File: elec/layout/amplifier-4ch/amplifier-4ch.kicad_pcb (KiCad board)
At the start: 2 copper layers, 9 parts, among them U1 240kΩ ±1% 62.5mW, U2 33kΩ ±1% 62.5mW, U3 240kΩ ±1% 62.5mW, U4 33kΩ ±1% 62.5mW, U5 240kΩ ±1% 62.5mW, U6 33kΩ ±1% 62.5mW, U7 240kΩ ±1% 62.5mW, U8 33kΩ ±1% 62.5mW

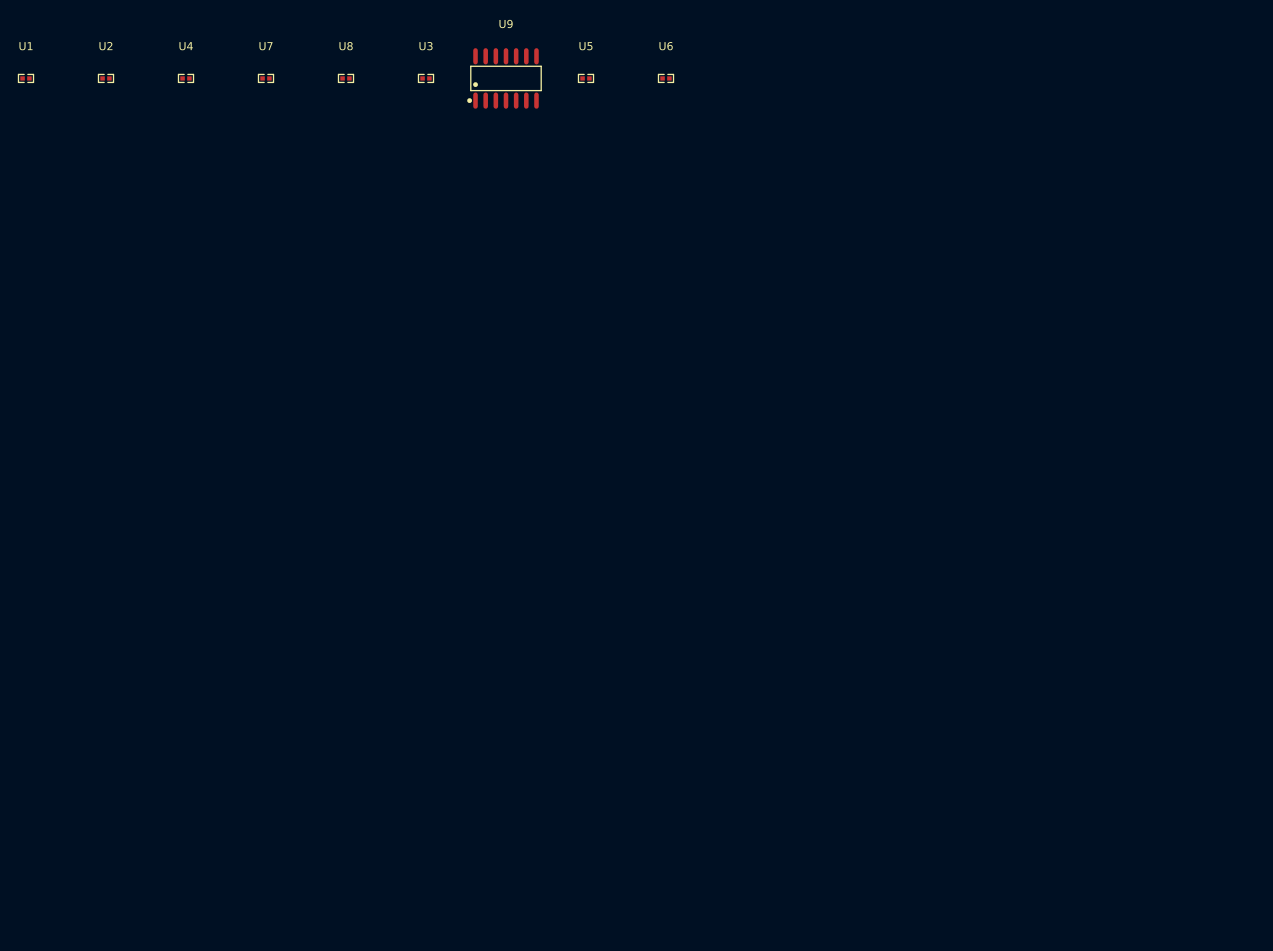
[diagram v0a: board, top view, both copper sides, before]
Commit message: Layout of amplifier-4ch
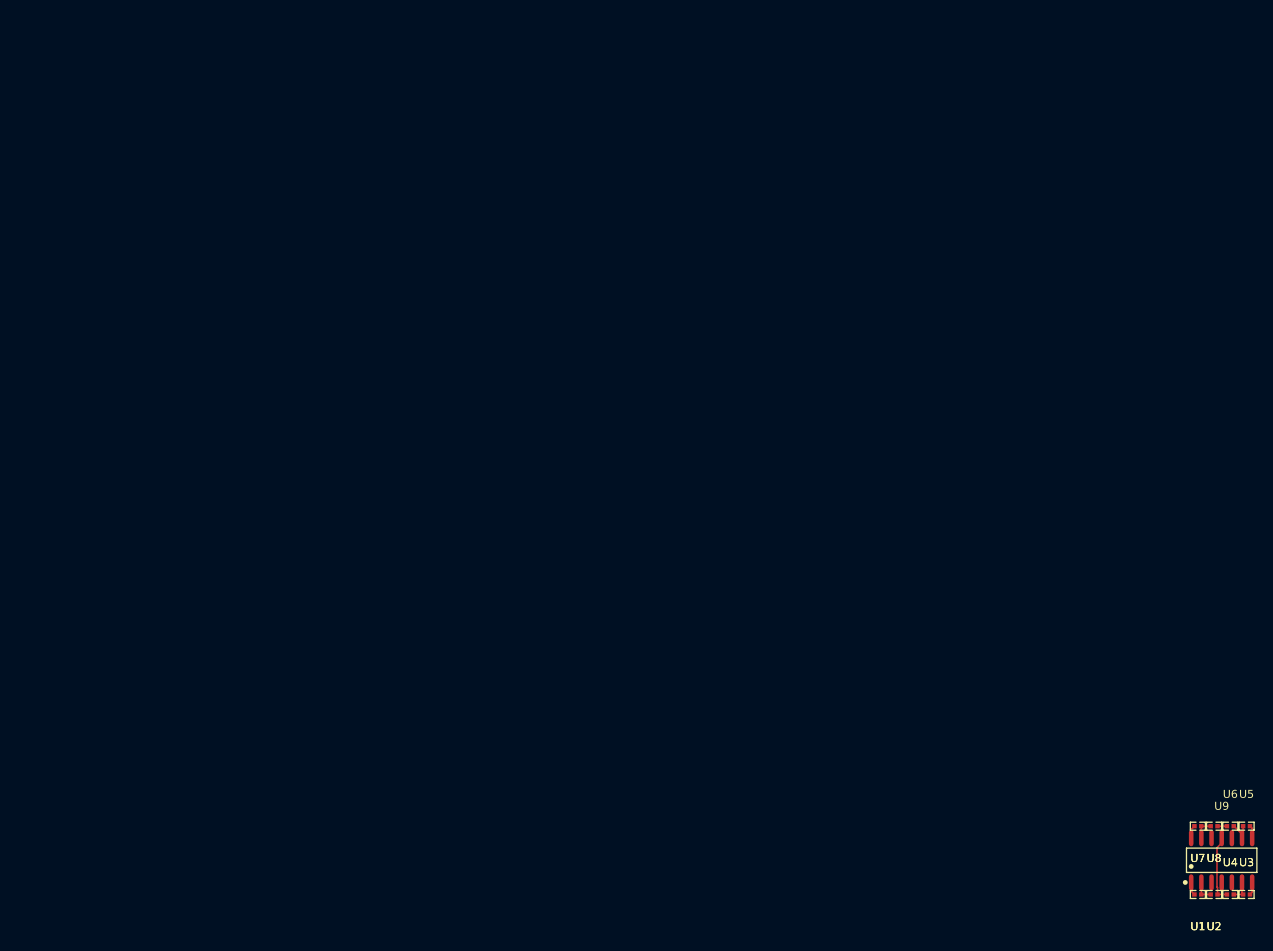
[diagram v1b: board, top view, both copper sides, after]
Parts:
- moved U1 178.5 mm to (156.5, 97.0), turned to 180 degrees
- moved U2 172.0 mm to (158.5, 97.0), turned to 180 degrees
- moved U4 165.7 mm to (160.5, 97.0)
- moved U7 149.3 mm to (156.5, 88.5), turned to 180 degrees
- moved U3 144.7 mm to (162.6, 97.0)
- moved U8 143.2 mm to (158.5, 88.5), turned to 180 degrees
- moved U9 132.5 mm to (159.5, 92.7)
- moved U5 124.7 mm to (162.6, 88.5)
- moved U6 117.1 mm to (160.5, 88.5)
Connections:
- net IN1_ renamed negative_terminal_1
- net IN1plus renamed input_1
- net IN2_ renamed negative_terminal_2
- net IN2plus renamed input_2
- net IN3_ renamed negative_terminal_3
- net IN4_ renamed negative_terminal_4
- net IN4plus renamed input_4
- net line renamed output_terminal_1
- net line-1 renamed output_terminal_2
- net line-2 renamed input_3
- net line-3 renamed output_terminal_4
- net line-4 renamed output_terminal_3
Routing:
- net gnd: track 0.00 -> 12.1 mm
- net negative_terminal_3: track 0.00 -> 3.49 mm
- net negative_terminal_2: track 0.00 -> 3.40 mm
- net negative_terminal_1: track 0.00 -> 3.18 mm
- net negative_terminal_4: track 0.00 -> 2.66 mm
- net output_terminal_4: track 0.00 -> 2.18 mm
- net output_terminal_1: track 0.00 -> 2.17 mm
- net output_terminal_2: track 0.00 -> 2.11 mm
- net output_terminal_3: track 0.00 -> 1.60 mm

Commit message: update syntax, delete vendored packages
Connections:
- net input_1 renamed IN1plus
- net input_2 renamed IN2plus
- net input_3 renamed IN3plus
- net input_4 renamed IN4plus
- net negative_terminal_1 renamed IN1_
- net negative_terminal_2 renamed IN2_
- net negative_terminal_3 renamed IN3_
- net negative_terminal_4 renamed IN4_
- net output_terminal_1 renamed line-2
- net output_terminal_2 renamed line-1
- net output_terminal_3 renamed line
- net output_terminal_4 renamed line-3

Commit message: build and re-link layouts
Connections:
- U3 pad 2: line-1 -> line
- U5 pad 2: line -> line-1
- U9 pad 7: line-1 -> line
- U9 pad 8: line -> line-1
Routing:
- net line-1: track 2.11 -> 1.60 mm
- net line: track 1.60 -> 2.11 mm
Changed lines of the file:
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@@
     (net 3 "IN2plus")
     (net 4 "IN1plus")
-    (net 5 "line")
+    (net 5 "line-1")
     (net 6 "hv")
     (net 7 "IN4plus")
@@
     (net 11 "line-2")
     (net 12 "IN4_")
-    (net 13 "line-1")
+    (net 13 "line")
     (net 14 "IN1_")
     (footprint "atopile:R0402-56259e"
@@
             (layers "F.Cu" "F.Paste" "F.Mask")
             (remove_unused_layers no)
-            (net 13 "line-1"))
+            (net 13 "line"))
         (pad "8" smd oval
             (at 3.81 -2.77 0)
@@
             (layers "F.Cu" "F.Paste" "F.Mask")
             (remove_unused_layers no)
-            (net 5 "line"))
+            (net 5 "line-1"))
         (pad "9" smd oval
             (at 2.54 -2.77 0)
@@
             (layers "F.Cu" "F.Paste" "F.Mask")
             (remove_unused_layers no)
-            (net 5 "line")))
+            (net 5 "line-1")))
     (footprint "atopile:R0402-56259e"
         (layer "F.Cu")
@@
             (layers "F.Cu" "F.Paste" "F.Mask")
             (remove_unused_layers no)
-            (net 13 "line-1")))
+            (net 13 "line")))
     (segment
         (start 162.139999 89.820001)

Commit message: all modules building
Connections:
- net IN1plus renamed line-4
- U1 pad 2: line-2 -> line-3
- U5 pad 2: line-1 -> line-2
- U7 pad 2: line-3 -> line-5
- U9 pad 1: line-2 -> line-3
- U9 pad 14: line-3 -> line-5
- U9 pad 5: IN2plus -> line-1
- U9 pad 8: line-1 -> line-2
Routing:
- net line-5: track 0.00 -> 2.18 mm
- net line-1: track 1.60 -> 0.00 mm
- net line-2: track 2.17 -> 1.60 mm
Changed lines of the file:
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@@
     (net 1 "IN3_")
     (net 2 "IN3plus")
-    (net 3 "IN2plus")
-    (net 4 "IN1plus")
-    (net 5 "line-1")
+    (net 3 "line-1")
+    (net 4 "line-4")
+    (net 5 "line-2")
     (net 6 "hv")
     (net 7 "IN4plus")
     (net 8 "gnd")
-    (net 9 "line-3")
+    (net 9 "line-5")
     (net 10 "IN2_")
-    (net 11 "line-2")
+    (net 11 "line-3")
     (net 12 "IN4_")
     (net 13 "line")
@@
                     (size 0.125 0.125)
                     (thickness 0.01875))))
-        (property "LCSC" "C64043"
-            (at 0 0 360)
-            (layer "User.9")
-            (hide yes)
-            (effects
-                (font
-                    (size 0.125 0.125)
-                    (thickness 0.01875))))
-        (property "Partnumber" "0402WGF2403TCE"
-            (at 0 0 360)
-            (layer "User.9")
-            (hide yes)
-            (effects
-                (font
-                    (size 0.125 0.125)
-                    (thickness 0.01875))))
-        (property "Manufacturer" "UNI-ROYAL(Uniroyal Elec)"
-            (at 0 0 360)
-            (layer "User.9")
-            (hide yes)
-            (effects
-                (font
-                    (size 0.125 0.125)
-                    (thickness 0.01875))))
-        (property "JLCPCB description" "62.5mW Thick Film Resistors 50V ±100ppm/℃ ±1% 240kΩ 0402 Chip Resistor - Surface Mount ROHS"
+        (property "LCSC" "C2909338"
+            (at 0 0 360)
+            (layer "User.9")
+            (hide yes)
+            (effects
+                (font
+                    (size 0.125 0.125)
+                    (thickness 0.01875))))
+        (property "Partnumber" "FRC0402F2403TS"
+            (at 0 0 360)
+            (layer "User.9")
+            (hide yes)
+            (effects
+                (font
+                    (size 0.125 0.125)
+                    (thickness 0.01875))))
+        (property "Manufacturer" "FOJAN"
+            (at 0 0 360)
+            (layer "User.9")
+            (hide yes)
+            (effects
+                (font
+                    (size 0.125 0.125)
+                    (thickness 0.01875))))
+        (property "JLCPCB description" "62.5mW Thick Film Resistors 50V ±100ppm/℃ ±1% 240kΩ 0402  Chip Resistor - Surface Mount ROHS"
             (at 0 0 360)
             (layer "User.9")
@@
             (layers "F.Cu" "F.Paste" "F.Mask")
             (remove_unused_layers no)
-            (net 9 "line-3")))
+            (net 9 "line-5")))
     (footprint "atopile:R0402-56259e"
         (layer "F.Cu")
@@
                     (size 0.125 0.125)
                     (thickness 0.01875))))
-        (property "LCSC" "C64043"
-            (at 0 0 360)
-            (layer "User.9")
-            (hide yes)
-            (effects
-                (font
-                    (size 0.125 0.125)
-                    (thickness 0.01875))))
-        (property "Partnumber" "0402WGF2403TCE"
-            (at 0 0 360)
-            (layer "User.9")
-            (hide yes)
-            (effects
-                (font
-                    (size 0.125 0.125)
-                    (thickness 0.01875))))
-        (property "Manufacturer" "UNI-ROYAL(Uniroyal Elec)"
-            (at 0 0 360)
-            (layer "User.9")
-            (hide yes)
-            (effects
-                (font
-                    (size 0.125 0.125)
-                    (thickness 0.01875))))
-        (property "JLCPCB description" "62.5mW Thick Film Resistors 50V ±100ppm/℃ ±1% 240kΩ 0402 Chip Resistor - Surface Mount ROHS"
+        (property "LCSC" "C2909338"
+            (at 0 0 360)
+            (layer "User.9")
+            (hide yes)
+            (effects
+                (font
+                    (size 0.125 0.125)
+                    (thickness 0.01875))))
+        (property "Partnumber" "FRC0402F2403TS"
+            (at 0 0 360)
+            (layer "User.9")
+            (hide yes)
+            (effects
+                (font
+                    (size 0.125 0.125)
+                    (thickness 0.01875))))
+        (property "Manufacturer" "FOJAN"
+            (at 0 0 360)
+            (layer "User.9")
+            (hide yes)
+            (effects
+                (font
+                    (size 0.125 0.125)
+                    (thickness 0.01875))))
+        (property "JLCPCB description" "62.5mW Thick Film Resistors 50V ±100ppm/℃ ±1% 240kΩ 0402  Chip Resistor - Surface Mount ROHS"
             (at 0 0 360)
             (layer "User.9")
@@
             (layers "F.Cu" "F.Paste" "F.Mask")
             (remove_unused_layers no)
-            (net 11 "line-2")))
+            (net 11 "line-3")))
     (footprint "atopile:R0402-56259e"
         (layer "F.Cu")
@@
             (layers "F.Cu" "F.Paste" "F.Mask")
             (remove_unused_layers no)
-            (net 11 "line-2"))
+            (net 11 "line-3"))
         (pad "2" smd oval
             (at -2.54 2.77 0)
@@
             (layers "F.Cu" "F.Paste" "F.Mask")
             (remove_unused_layers no)
-            (net 4 "IN1plus"))
+            (net 4 "line-4"))
         (pad "4" smd oval
             (at 0 2.77 0)
@@
             (layers "F.Cu" "F.Paste" "F.Mask")
             (remove_unused_layers no)
-            (net 3 "IN2plus"))
+            (net 3 "line-1"))
         (pad "6" smd oval
             (at 2.54 2.77 0)
@@
             (layers "F.Cu" "F.Paste" "F.Mask")
             (remove_unused_layers no)
-            (net 5 "line-1"))
+            (net 5 "line-2"))
         (pad "9" smd oval
             (at 2.54 -2.77 0)
@@
             (layers "F.Cu" "F.Paste" "F.Mask")
             (remove_unused_layers no)
-            (net 9 "line-3")))
+            (net 9 "line-5")))
     (footprint "atopile:R0402-56259e"
         (layer "F.Cu")
@@
                     (size 0.125 0.125)
                     (thickness 0.01875))))
-        (property "LCSC" "C64043"
-            (at 0 0 0)
-            (layer "User.9")
-            (hide yes)
-            (effects
-                (font
-                    (size 0.125 0.125)
-                    (thickness 0.01875))))
-        (property "Partnumber" "0402WGF2403TCE"
-            (at 0 0 0)
-            (layer "User.9")
-            (hide yes)
-            (effects
-                (font
-                    (size 0.125 0.125)
-                    (thickness 0.01875))))
-        (property "Manufacturer" "UNI-ROYAL(Uniroyal Elec)"
-            (at 0 0 0)
-            (layer "User.9")
-            (hide yes)
-            (effects
-                (font
-                    (size 0.125 0.125)
-                    (thickness 0.01875))))
-        (property "JLCPCB description" "62.5mW Thick Film Resistors 50V ±100ppm/℃ ±1% 240kΩ 0402 Chip Resistor - Surface Mount ROHS"
+        (property "LCSC" "C2909338"
+            (at 0 0 0)
+            (layer "User.9")
+            (hide yes)
+            (effects
+                (font
+                    (size 0.125 0.125)
+                    (thickness 0.01875))))
+        (property "Partnumber" "FRC0402F2403TS"
+            (at 0 0 0)
+            (layer "User.9")
+            (hide yes)
+            (effects
+                (font
+                    (size 0.125 0.125)
+                    (thickness 0.01875))))
+        (property "Manufacturer" "FOJAN"
+            (at 0 0 0)
+            (layer "User.9")
+            (hide yes)
+            (effects
+                (font
+                    (size 0.125 0.125)
+                    (thickness 0.01875))))
+        (property "JLCPCB description" "62.5mW Thick Film Resistors 50V ±100ppm/℃ ±1% 240kΩ 0402  Chip Resistor - Surface Mount ROHS"
             (at 0 0 0)
             (layer "User.9")
@@
             (layers "F.Cu" "F.Paste" "F.Mask")
             (remove_unused_layers no)
-            (net 5 "line-1")))
+            (net 5 "line-2")))
     (footprint "atopile:R0402-56259e"
         (layer "F.Cu")
@@
                     (size 0.125 0.125)
                     (thickness 0.01875))))
-        (property "LCSC" "C64043"
-            (at 0 0 0)
-            (layer "User.9")
-            (hide yes)
-            (effects
-                (font
-                    (size 0.125 0.125)
-                    (thickness 0.01875))))
-        (property "Partnumber" "0402WGF2403TCE"
-            (at 0 0 0)
-            (layer "User.9")
-            (hide yes)
-            (effects
-                (font
-                    (size 0.125 0.125)
-                    (thickness 0.01875))))
-        (property "Manufacturer" "UNI-ROYAL(Uniroyal Elec)"
-            (at 0 0 0)
-            (layer "User.9")
-            (hide yes)
-            (effects
-                (font
-                    (size 0.125 0.125)
-                    (thickness 0.01875))))
-        (property "JLCPCB description" "62.5mW Thick Film Resistors 50V ±100ppm/℃ ±1% 240kΩ 0402 Chip Resistor - Surface Mount ROHS"
-            (at 0 0 0)
-            (layer "User.9")
+        (property "LCSC" "C2909338"
+            (at 0 0 0)
+            (layer "User.9")
+            (hide yes)
+            (effects
+                (font
+                    (size 0.125 0.125)
+                    (thickness 0.01875))))
+        (property "Partnumber" "FRC0402F2403TS"
+            (at 0 0 0)
+            (layer "User.9")
+            (hide yes)
+            (effects
+                (font
+                    (size 0.125 0.125)
+                    (thickness 0.01875))))
+        (property "Manufacturer" "FOJAN"
+            (at 0 0 0)
+            (layer "User.9")
+            (hide yes)
+            (effects
+                (font
+                    (size 0.125 0.125)
+                    (thickness 0.01875))))
+        (property "JLCPCB description" "62.5mW Thick Film Resistors 50V ±100ppm/℃ ±1% 240kΩ 0402  Chip Resistor - Surface Mount ROHS"
+            (at 0 0 0)
+            (layer "User.9")

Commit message: HIL Building
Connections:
- net line-4 renamed IN1plus
- U1 pad 2: line-3 -> line
- U3 pad 2: line -> line-1
- U7 pad 2: line-5 -> line-3
- U9 pad 1: line-3 -> line
- U9 pad 14: line-5 -> line-3
- U9 pad 5: line-1 -> IN2plus
- U9 pad 7: line -> line-1
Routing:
- net line-5: track 2.18 -> 0.00 mm
- net line-1: track 0.00 -> 2.11 mm
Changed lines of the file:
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@@
     (net 1 "IN3_")
     (net 2 "IN3plus")
-    (net 3 "line-1")
-    (net 4 "line-4")
+    (net 3 "IN2plus")
+    (net 4 "IN1plus")
     (net 5 "line-2")
     (net 6 "hv")
     (net 7 "IN4plus")
     (net 8 "gnd")
-    (net 9 "line-5")
+    (net 9 "line-3")
     (net 10 "IN2_")
-    (net 11 "line-3")
+    (net 11 "line")
     (net 12 "IN4_")
-    (net 13 "line")
+    (net 13 "line-1")
     (net 14 "IN1_")
     (footprint "atopile:R0402-56259e"
@@
             (layers "F.Cu" "F.Paste" "F.Mask")
             (remove_unused_layers no)
-            (net 9 "line-5")))
+            (net 9 "line-3")))
     (footprint "atopile:R0402-56259e"
         (layer "F.Cu")
@@
             (layers "F.Cu" "F.Paste" "F.Mask")
             (remove_unused_layers no)
-            (net 11 "line-3")))
+            (net 11 "line")))
     (footprint "atopile:R0402-56259e"
         (layer "F.Cu")
@@
             (layers "F.Cu" "F.Paste" "F.Mask")
             (remove_unused_layers no)
-            (net 11 "line-3"))
+            (net 11 "line"))
         (pad "2" smd oval
             (at -2.54 2.77 0)
@@
             (layers "F.Cu" "F.Paste" "F.Mask")
             (remove_unused_layers no)
-            (net 4 "line-4"))
+            (net 4 "IN1plus"))
         (pad "4" smd oval
             (at 0 2.77 0)
@@
             (layers "F.Cu" "F.Paste" "F.Mask")
             (remove_unused_layers no)
-            (net 3 "line-1"))
+            (net 3 "IN2plus"))
         (pad "6" smd oval
             (at 2.54 2.77 0)
@@
             (layers "F.Cu" "F.Paste" "F.Mask")
             (remove_unused_layers no)
-            (net 13 "line"))
+            (net 13 "line-1"))
         (pad "8" smd oval
             (at 3.81 -2.77 0)
@@
             (layers "F.Cu" "F.Paste" "F.Mask")
             (remove_unused_layers no)
-            (net 9 "line-5")))
+            (net 9 "line-3")))
     (footprint "atopile:R0402-56259e"
         (layer "F.Cu")
@@
             (layers "F.Cu" "F.Paste" "F.Mask")
             (remove_unused_layers no)
-            (net 13 "line")))
+            (net 13 "line-1")))
     (segment
         (start 162.139999 89.820001)
